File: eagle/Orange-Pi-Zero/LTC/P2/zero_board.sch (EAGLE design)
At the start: 17 parts, among them IC1 MCP6002DIP

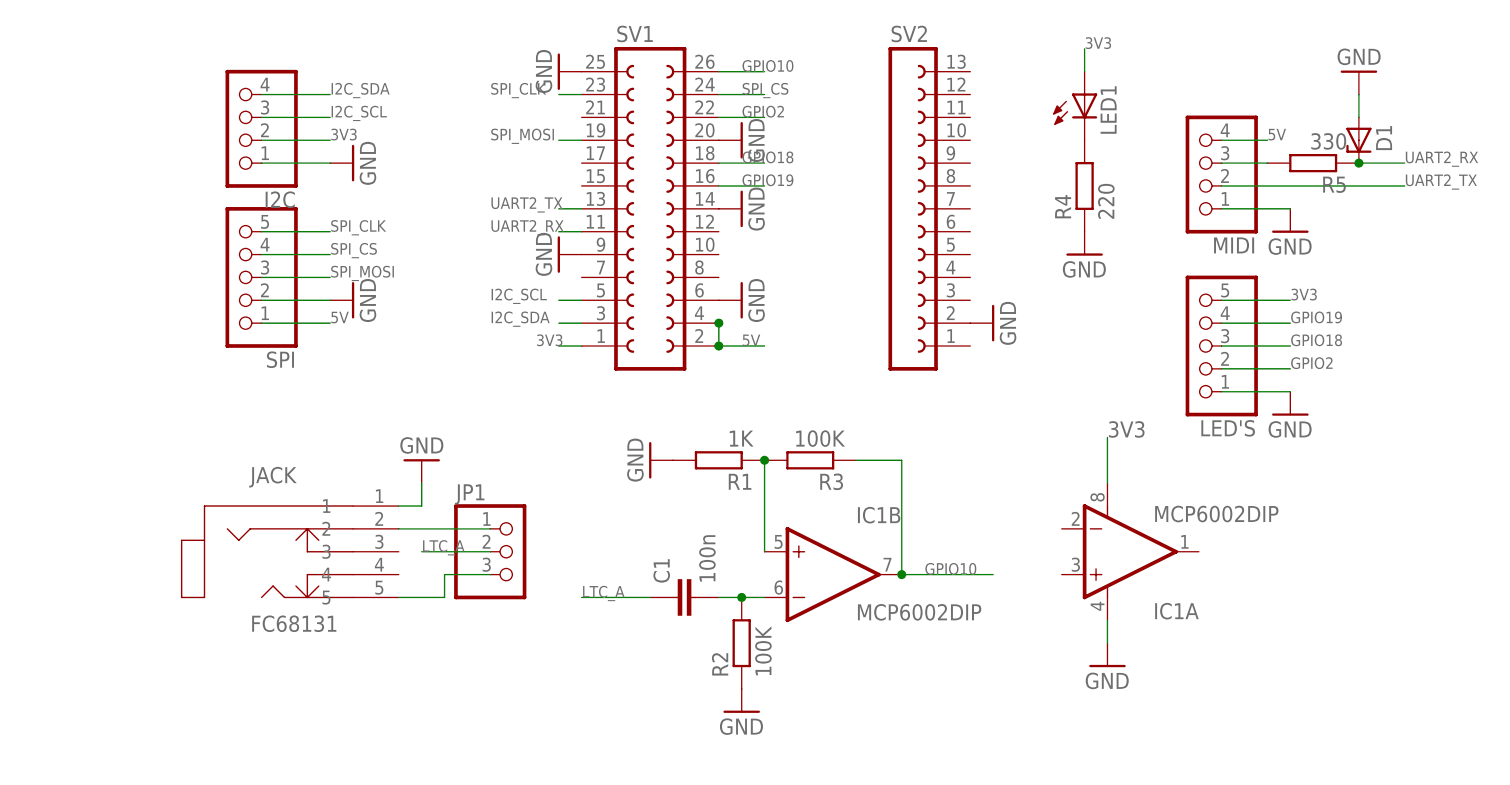
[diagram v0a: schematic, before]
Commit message: Added new gerber.zip files
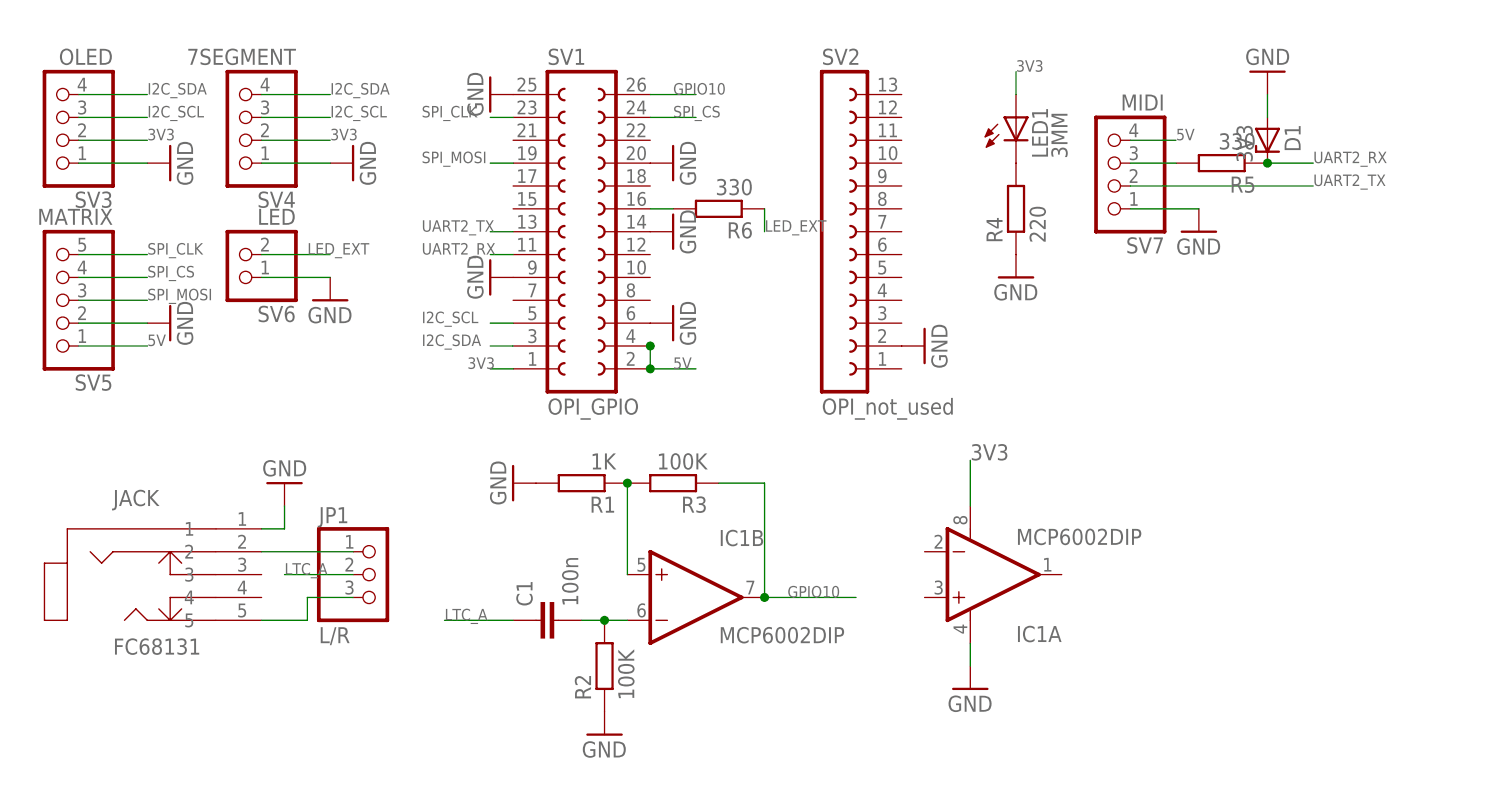
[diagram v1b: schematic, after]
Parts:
- removed LED'S, SPI: (no value), pinhead:PINHD-1X5
- removed MIDI: (no value), pinhead:PINHD-1X4
- added R6: 330, rcl:R-EU_0204/2V
- added SV3: OLED, pinhead:PINHD-1X4
- added SV5: MATRIX, pinhead:PINHD-1X5
- added SV6: LED, pinhead:PINHD-1X2
- added SV7: MIDI, pinhead:PINHD-1X4
- D1: value (none) -> 3V3
- JP1: value (none) -> L/R
- LED1: value (none) -> 3MM
- SV1: value (none) -> OPI_GPIO
- SV2: value (none) -> OPI_not_used
- SV4: value (none) -> 7SEGMENT
- renumbered I2C to SV4
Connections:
- removed net GPIO18: LED'S.3, SV1.18
- removed net GPIO19: LED'S.4, SV1.16
- removed net GPIO2: LED'S.2, SV1.22
- new net LED_EXT: R6.1, SV6.2
- new net N$4: R6.2, SV1.16
- net 3V3: now also SV3.2; no longer LED'S.5
- net 5V: now also SV5.1, SV7.4; no longer MIDI.4, SPI.1
- net GND: now also SV3.1, SV5.2, SV6.1, SV7.1; no longer LED'S.1, MIDI.1, SPI.2
- net I2C_SCL: now also SV3.3
- net I2C_SDA: now also SV3.4
- net N$7: now also SV7.3; no longer MIDI.3
- net SPI_CLK: now also SV5.5; no longer SPI.5
- net SPI_CS: now also SV5.4; no longer SPI.4
- net SPI_MOSI: now also SV5.3; no longer SPI.3
- net UART2_TX: now also SV7.2; no longer MIDI.2
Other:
- moved on the sheet: C1, D1, IC1A, IC1B, JACK, JP1, LED1, R1, R2, R3, R4, R5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
